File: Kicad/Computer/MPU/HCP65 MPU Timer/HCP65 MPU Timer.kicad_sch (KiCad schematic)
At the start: 20 parts, among them IC1 74LVC2G74DP,125, IC11 74LVC1G27GW,125, IC14 74HCT4040PW,118, IC2 74LVC273PW,118, IC5 AP7365-33WG-7, IC6 74HCT4040PW,118, IC7 PI3B3251QE, IC9 74LVC541APW,118, J1 Pin_Header_01x16, J2 Conn_02x16_Counter_Clockwise, J3 Pin_Header_01x16

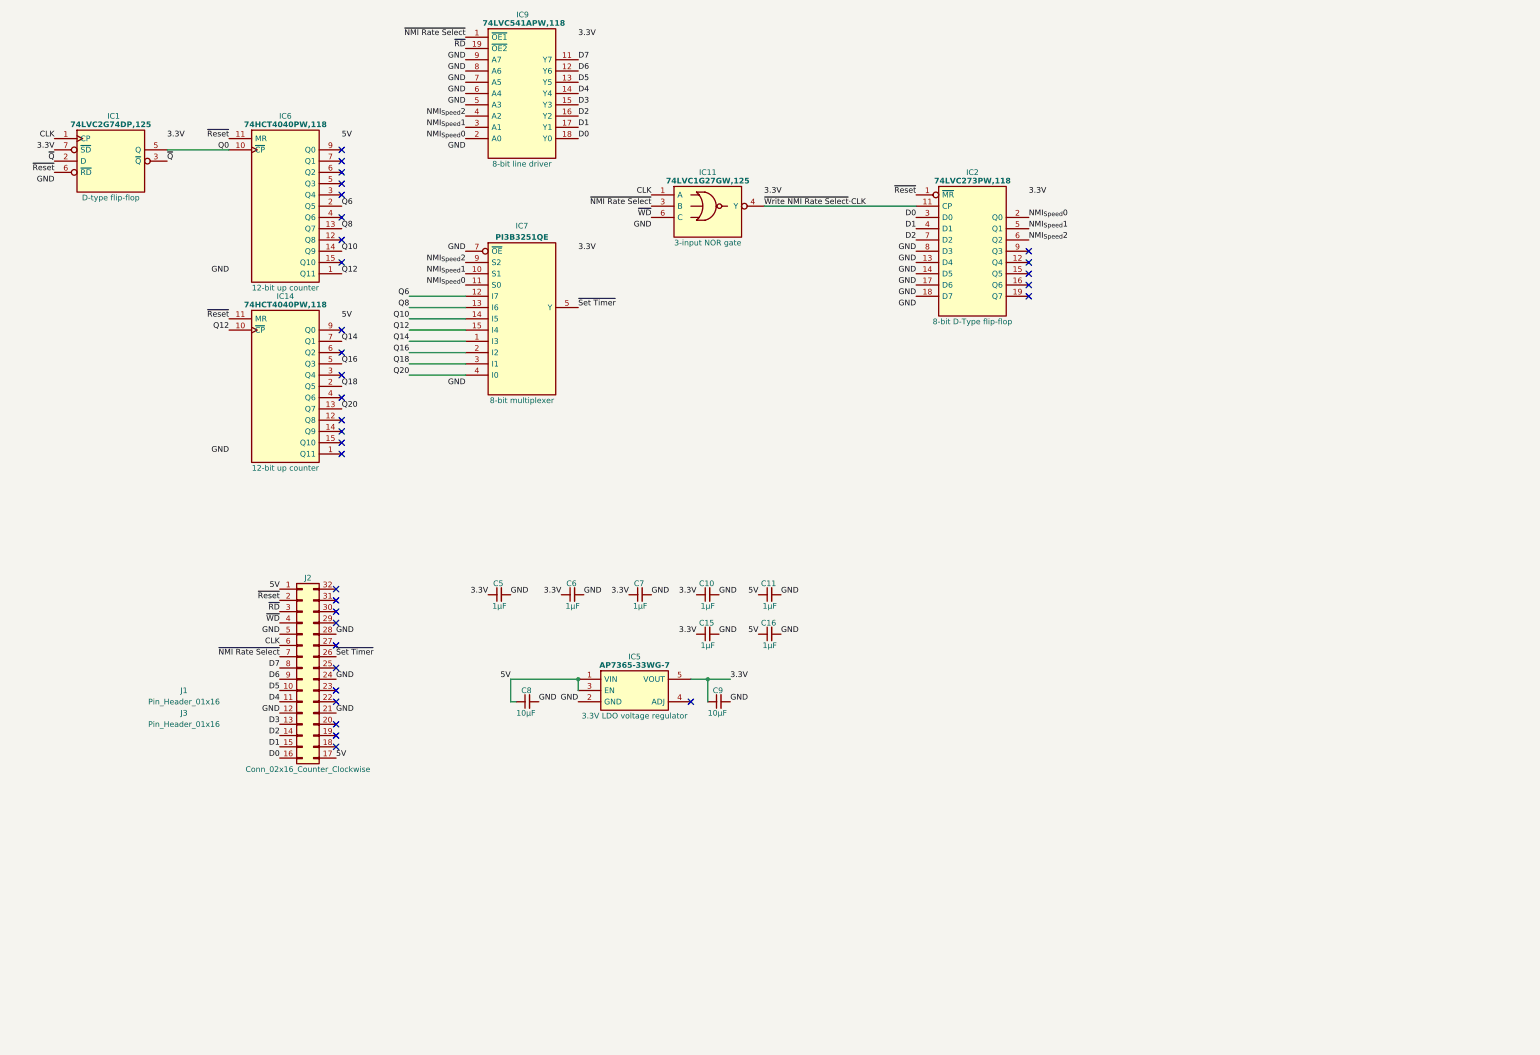
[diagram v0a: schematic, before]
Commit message: Generating MPU gerbers again with paste layers.
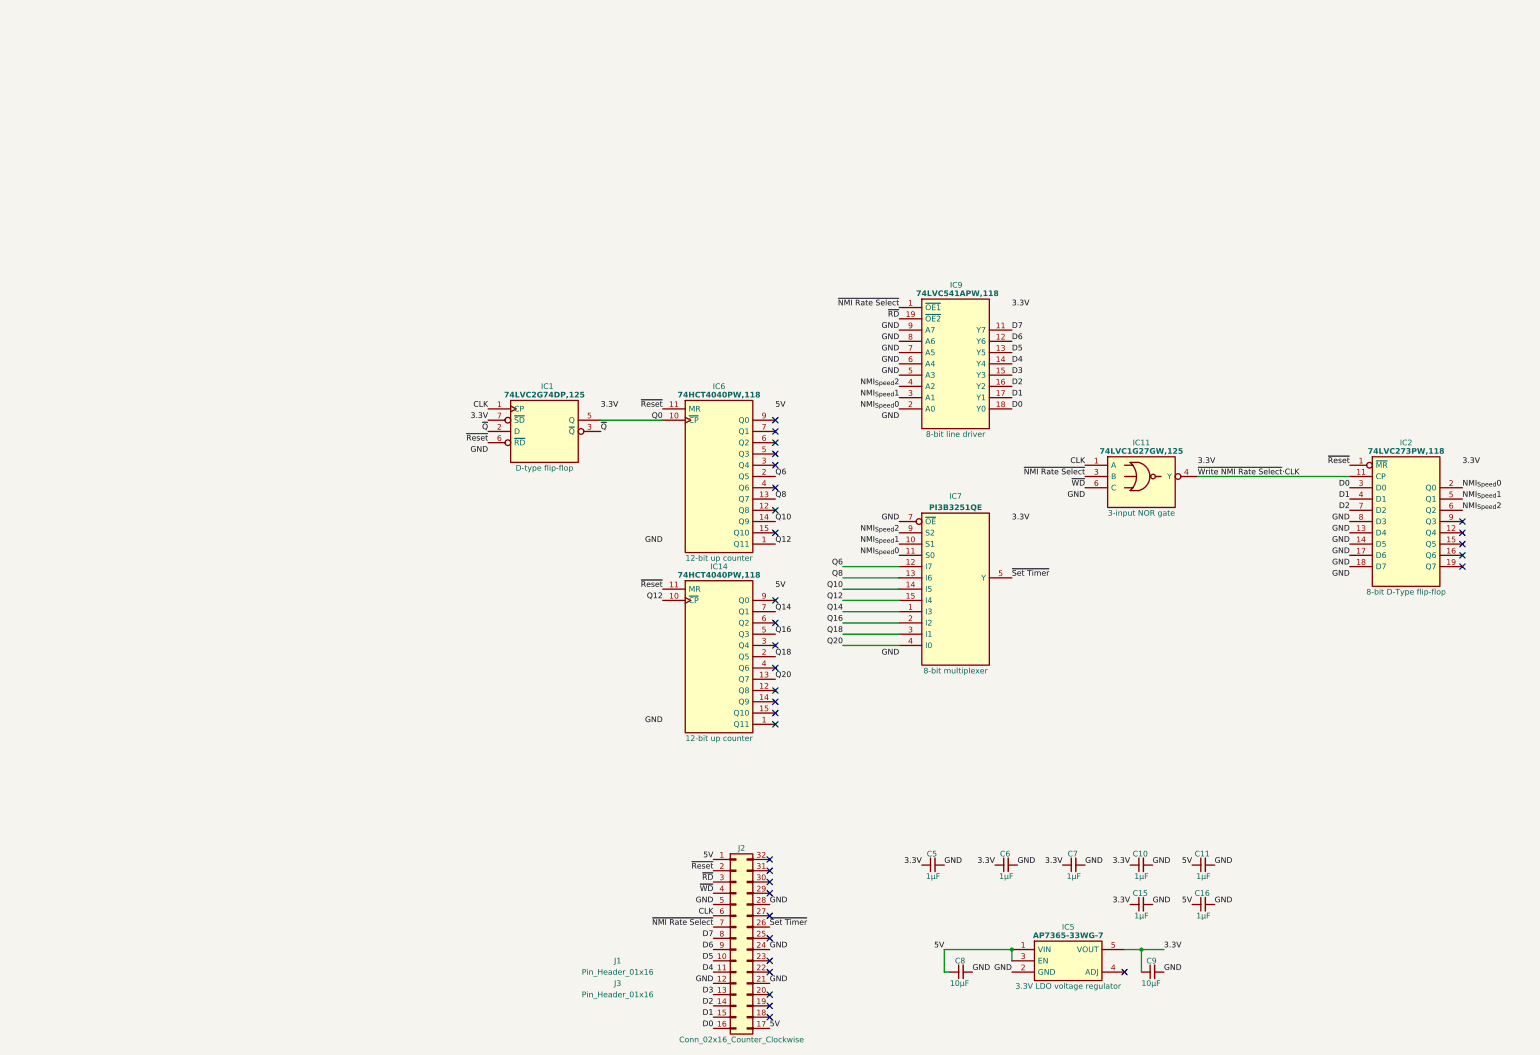
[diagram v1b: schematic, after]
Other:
- moved on the sheet: C10, C11, C15, C16, C5, C6, C7, C8, C9, IC1, IC11, IC14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

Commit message: Re-autorouted a bunch of boards.  Or something.  I don't know.
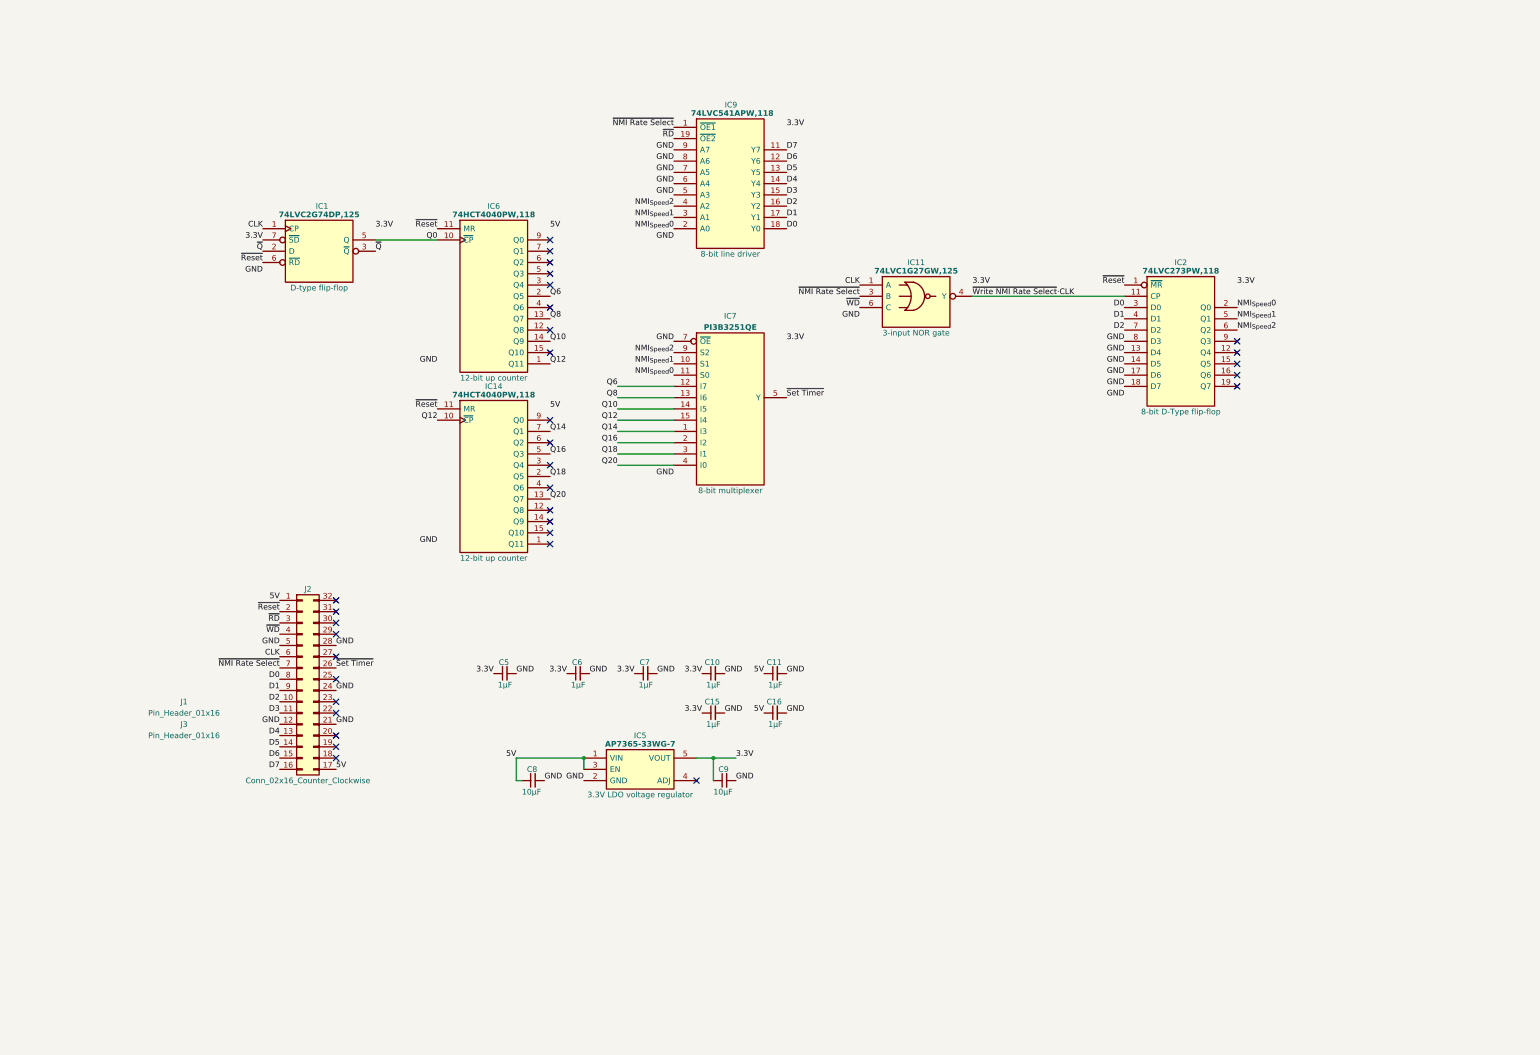
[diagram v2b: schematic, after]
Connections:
- net D0: now also J2.8 (Pin_8); no longer J2.16 (Pin_16)
- net D1: now also J2.9 (Pin_9); no longer J2.15 (Pin_15)
- net D2: now also J2.10 (Pin_10); no longer J2.14 (Pin_14)
- net D3: now also J2.11 (Pin_11); no longer J2.13 (Pin_13)
- net D4: now also J2.13 (Pin_13); no longer J2.11 (Pin_11)
- net D5: now also J2.14 (Pin_14); no longer J2.10 (Pin_10)
- net D6: now also J2.15 (Pin_15); no longer J2.9 (Pin_9)
- net D7: now also J2.16 (Pin_16); no longer J2.8 (Pin_8)
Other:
- moved on the sheet: C10, C11, C15, C16, C5, C6, C7, C8, C9, IC1, IC11, IC14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
